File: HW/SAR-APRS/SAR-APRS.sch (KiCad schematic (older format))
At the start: 0 parts

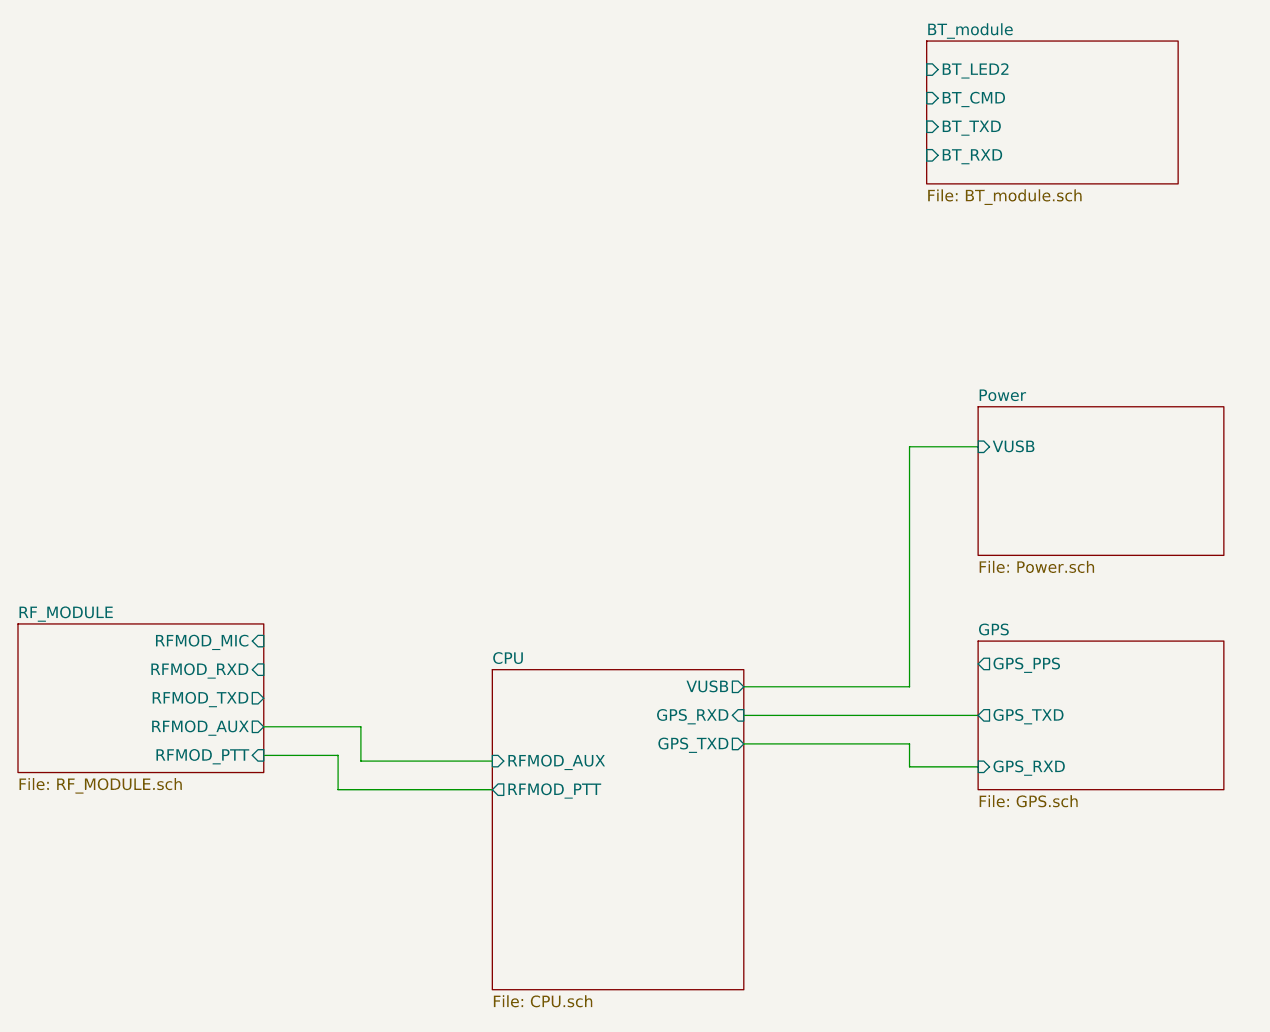
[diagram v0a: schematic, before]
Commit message: schem and pcb update
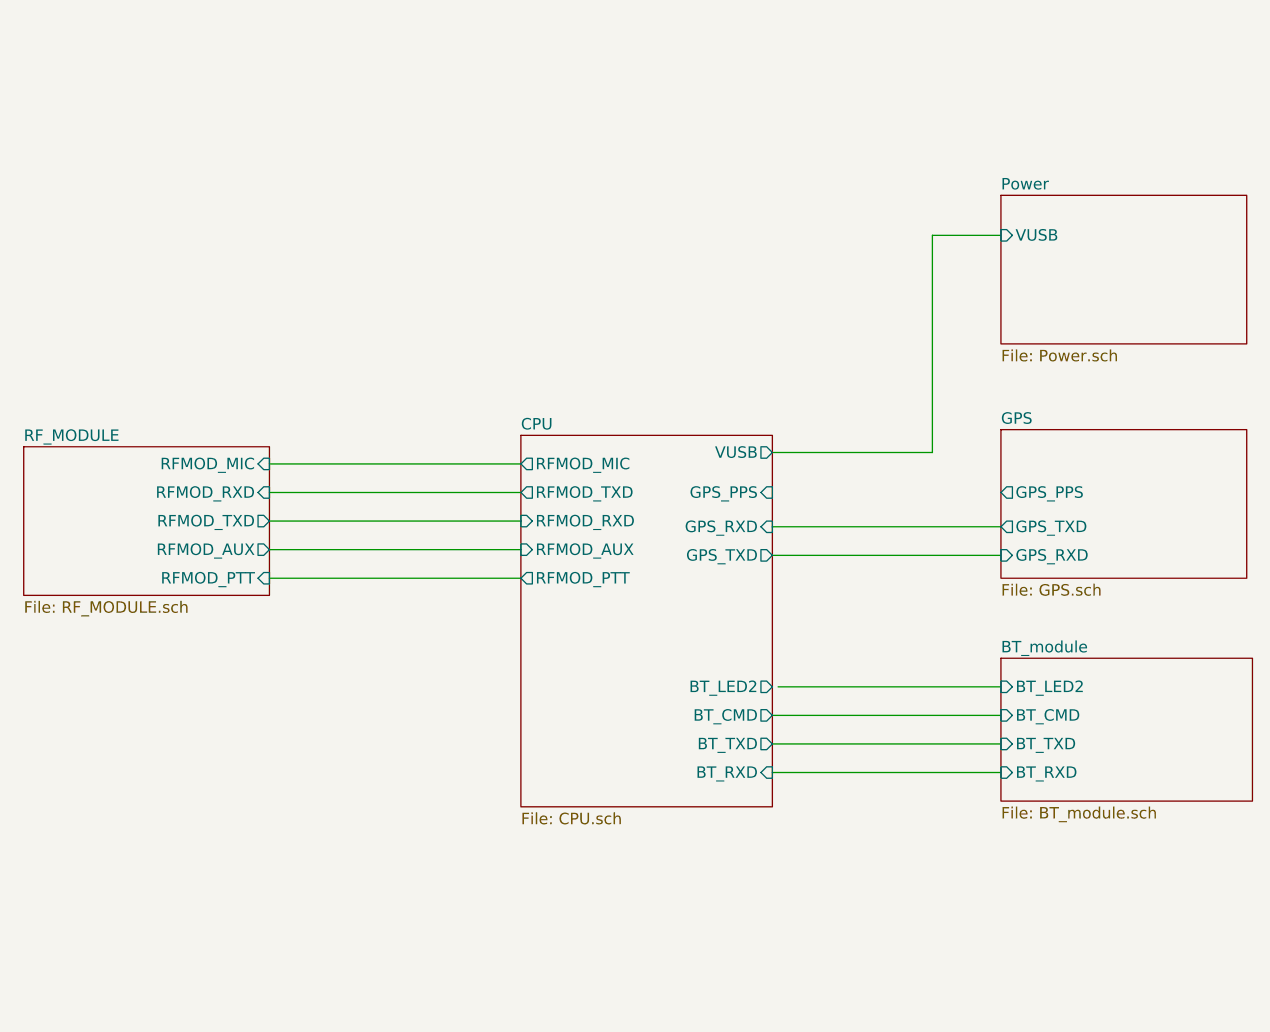
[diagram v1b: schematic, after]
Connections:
- wire segments 13 -> 14
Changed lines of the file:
@@
 EESchema Schematic File Version 4
 LIBS:SAR-APRS-cache
-EELAYER 28 0
+EELAYER 29 0
 EELAYER END
 $Descr A3 16535 11693
@@
 $EndDescr
 $Sheet
-S 5350 5775 1075 650
+S 5375 5000 1075 650
 U 5C8B81A5
 F0 "RF_MODULE" 50
 F1 "RF_MODULE.sch" 50
-F2 "RFMOD_MIC" I R 6425 5850 50
-F3 "RFMOD_RXD" I R 6425 5975 50
-F4 "RFMOD_TXD" O R 6425 6100 50
-F5 "RFMOD_AUX" O R 6425 6225 50
-F6 "RFMOD_PTT" I R 6425 6350 50
+F2 "RFMOD_MIC" I R 6450 5075 50
+F3 "RFMOD_RXD" I R 6450 5200 50
+F4 "RFMOD_TXD" O R 6450 5325 50
+F5 "RFMOD_AUX" O R 6450 5450 50
+F6 "RFMOD_PTT" I R 6450 5575 50
 $EndSheet
 $Sheet
-S 9550 4825 1075 650
+S 9650 3900 1075 650
 U 5C948828
 F0 "Power" 50
 F1 "Power.sch" 50
-F2 "VUSB" I L 9550 5000 50
+F2 "VUSB" I L 9650 4075 50
 $EndSheet
 $Sheet
-S 7425 5975 1100 1400
+S 7550 4950 1100 1625
 U 5CB07977
 F0 "CPU" 50
 F1 "CPU.sch" 50
-F2 "GPS_RXD" I R 8525 6175 50
-F3 "GPS_TXD" O R 8525 6300 50
-F4 "RFMOD_PTT" O L 7425 6500 50
-F5 "RFMOD_AUX" I L 7425 6375 50
-F6 "VUSB" O R 8525 6050 50
+F2 "GPS_RXD" I R 8650 5350 50
+F3 "GPS_TXD" O R 8650 5475 50
+F4 "RFMOD_PTT" O L 7550 5575 50
+F5 "RFMOD_AUX" I L 7550 5450 50
+F6 "VUSB" O R 8650 5025 50
+F7 "RFMOD_TXD" O L 7550 5200 50
+F8 "RFMOD_RXD" I L 7550 5325 50
+F9 "RFMOD_MIC" O L 7550 5075 50
+F10 "GPS_PPS" I R 8650 5200 50
+F11 "BT_TXD" O R 8650 6300 50
+F12 "BT_RXD" I R 8650 6425 50
+F13 "BT_LED2" O R 8650 6050 50
+F14 "BT_CMD" O R 8650 6175 50
 $EndSheet
 $Sheet
-S 9325 3225 1100 625
+S 9650 5925 1100 625
 U 5C81D1BC
 F0 "BT_module" 50
 F1 "BT_module.sch" 50
-F2 "BT_LED2" I L 9325 3350 50
-F3 "BT_CMD" I L 9325 3475 50
-F4 "BT_TXD" I L 9325 3600 50
-F5 "BT_RXD" I L 9325 3725 50
+F2 "BT_LED2" I L 9650 6050 50
+F3 "BT_CMD" I L 9650 6175 50
+F4 "BT_TXD" I L 9650 6300 50
+F5 "BT_RXD" I L 9650 6425 50
 $EndSheet
 $Sheet
-S 9550 5850 1075 650
+S 9650 4925 1075 650
 U 5C97B601
 F0 "GPS" 50
 F1 "GPS.sch" 50
-F2 "GPS_PPS" O L 9550 5950 50
-F3 "GPS_TXD" O L 9550 6175 50
-F4 "GPS_RXD" I L 9550 6400 50
+F2 "GPS_PPS" O L 9650 5200 50
+F3 "GPS_TXD" O L 9650 5350 50
+F4 "GPS_RXD" I L 9650 5475 50
 $EndSheet
 Wire Wire Line
-	9550 6175 8525 6175
+	9650 5350 8650 5350
 Wire Wire Line
-	8525 6300 9250 6300
+	8650 5025 9350 5025
 Wire Wire Line
-	9250 6300 9250 6400
+	9350 5025 9350 4075
 Wire Wire Line
-	9250 6400 9550 6400
+	9350 4075 9650 4075
 Wire Wire Line
-	6425 6225 6850 6225
+	6450 5575 7550 5575
 Wire Wire Line
-	6850 6225 6850 6375
+	6450 5450 7550 5450
 Wire Wire Line
-	6850 6375 7425 6375
+	6450 5325 7550 5325
 Wire Wire Line
-	6425 6350 6750 6350
+	6450 5200 7550 5200
 Wire Wire Line
-	6750 6350 6750 6500
+	7550 5075 6450 5075
 Wire Wire Line
-	6750 6500 7425 6500
+	8650 5475 9650 5475
 Wire Wire Line
-	8525 6050 9250 6050
+	8650 6425 9650 6425
 Wire Wire Line
-	9250 6050 9250 5000
+	8650 6300 9650 6300
 Wire Wire Line
-	9250 5000 9550 5000
+	8650 6175 9650 6175
+Wire Wire Line
+	8675 6050 9650 6050
 $EndSCHEMATC
